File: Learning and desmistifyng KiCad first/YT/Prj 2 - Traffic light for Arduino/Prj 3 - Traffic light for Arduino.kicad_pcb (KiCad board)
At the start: 2 copper layers, 36 x 50.5 mm, 11 parts, among them J2 Conn_01x04

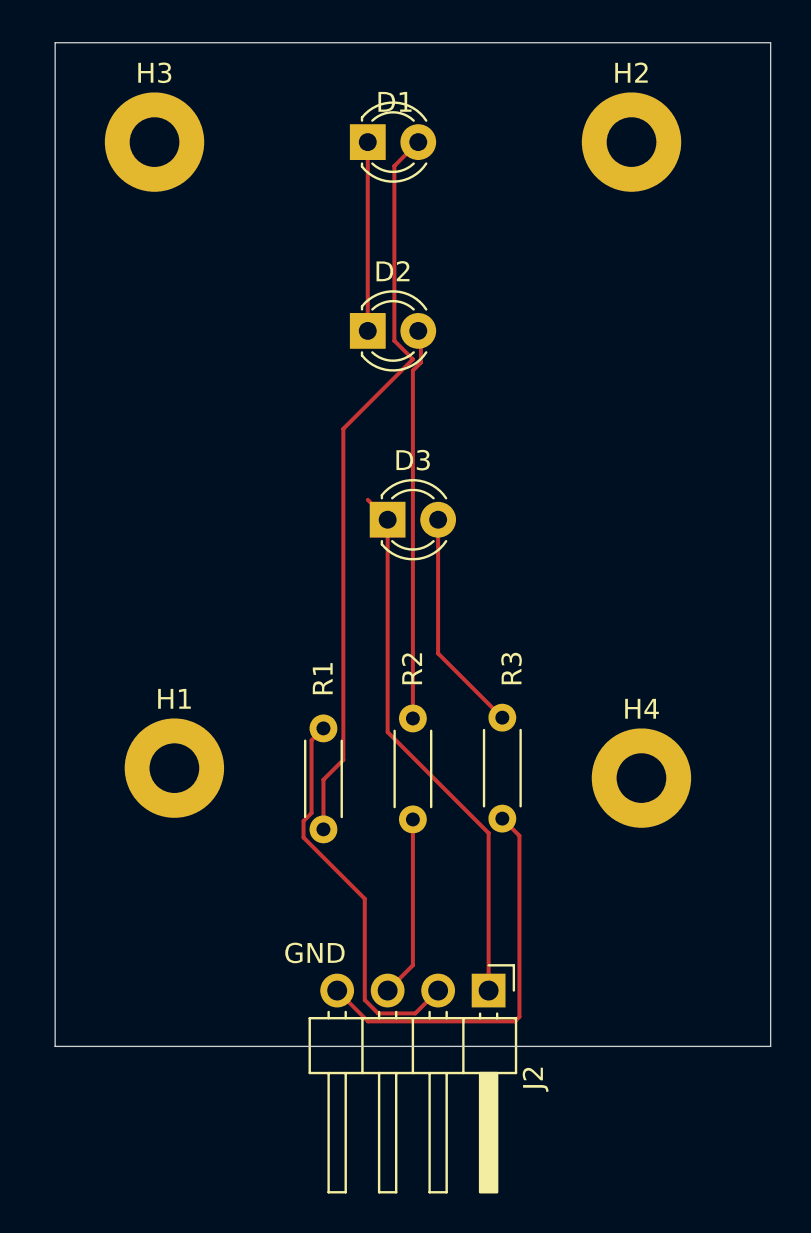
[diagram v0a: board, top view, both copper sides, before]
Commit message: updates on demistifying kicad
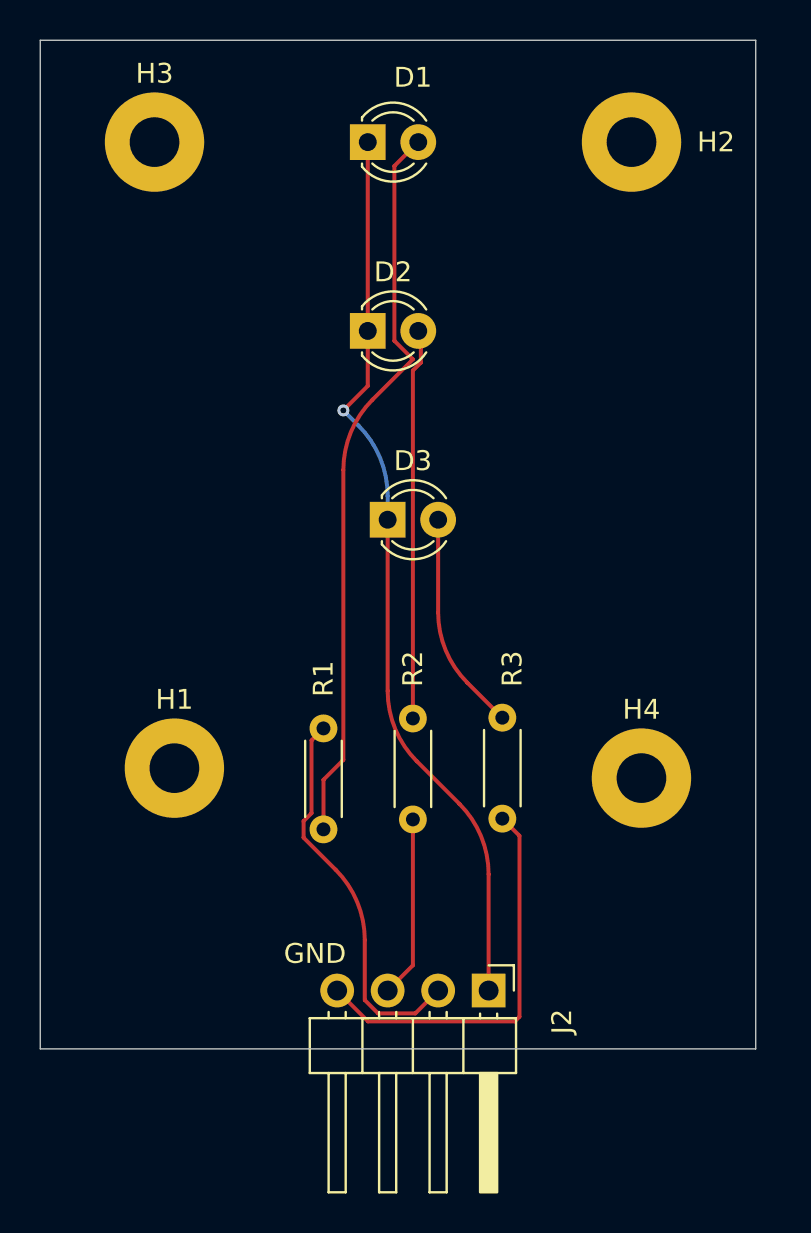
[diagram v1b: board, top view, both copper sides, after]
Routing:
- net Net-(D1-K): track 36.7 -> 45.5 mm, vias 0 -> 1
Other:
- board size 36 x 50.5 mm -> 36 x 50.8 mm
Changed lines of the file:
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@@
 		(tags "mountinghole")
 		(property "Reference" "H2"
-			(at 0 -3.45 0)
+			(at 4.25 0 0)
 			(layer "F.SilkS")
 			(effects
@@
 		)
 		(property "Value" "MountingHole"
-			(at 0 3.45 0)
+			(at 0.25 3.75 0)
 			(layer "F.Fab")
 			(effects
@@
 		)
 		(fp_text user "${REFERENCE}"
-			(at 0 0 0)
+			(at -3.25 2 0)
 			(layer "F.Fab")
 			(effects
@@
 		(tags "LED")
 		(property "Reference" "D1"
-			(at 1.36566 -1.987699 0)
+			(at 2.27 -3.25 0)
 			(layer "F.SilkS")
 			(effects
@@
 		(tags "Through hole angled pin header THT 1x04 2.54mm single row")
 		(property "Reference" "J2"
-			(at 4.385 -2.27 90)
+			(at 1.56 -3.69 90)
 			(layer "F.SilkS")
 			(effects
@@
 			)
 			(layer "F.Fab")
-		)
-		(fp_text user "${REFERENCE}"
-			(at 2.77 3.81 0)
-			(layer "F.Fab")
-			(effects
-				(font
-					(size 1 1)
-					(thickness 0.15)
-				)
-			)
 		)
 		(pad "1" thru_hole rect
@@
 	)
 	(gr_rect
-		(start 160 42.5)
-		(end 196 93)
+		(start 159.25 42.375)
+		(end 195.25 93.125)
 		(stroke
 			(width 0.05)
@@
 	)
 	(segment
-		(start 174.501 61.927471)
+		(start 175.965466 60.463005)
 		(end 178 58.428471)
 		(width 0.2)
@@
 	(segment
 		(start 174.501 78.583372)
-		(end 174.501 61.927471)
+		(end 174.501 63.998539)
 		(width 0.2)
 		(layer "F.Cu")
 		(net 1)
 	)
-	(segment
-		(start 181.81 82.265628)
-		(end 176.73 77.185628)
+	(arc
+		(start 174.501 63.998539)
+		(mid 174.881602 62.085122)
+		(end 175.965466 60.463005)
+		(width 0.2)
+		(layer "F.Cu")
+		(net 1)
+	)
+	(segment
+		(start 180.345534 80.801162)
+		(end 178.194466 78.650094)
 		(width 0.2)
 		(layer "F.Cu")
@@
 	)
 	(segment
-		(start 175.73 65.5)
+		(start 181.81 90.19)
+		(end 181.81 84.336696)
+		(width 0.2)
+		(layer "F.Cu")
+		(net 2)
+	)
+	(segment
+		(start 175.73 59.77)
+		(end 174.5 61)
+		(width 0.2)
+		(layer "F.Cu")
+		(net 2)
+	)
+	(segment
+		(start 175.73 57)
+		(end 175.73 59.77)
+		(width 0.2)
+		(layer "F.Cu")
+		(net 2)
+	)
+	(segment
+		(start 176.73 75.11456)
 		(end 176.73 66.5)
 		(width 0.2)
@@
 		(net 2)
 	)
-	(segment
-		(start 181.81 90.19)
-		(end 181.81 82.265628)
-		(width 0.2)
-		(layer "F.Cu")
+	(via
+		(at 174.5 61)
+		(size 0.6)
+		(drill 0.3)
+		(layers "F.Cu" "B.Cu")
 		(net 2)
 	)
-	(segment
-		(start 176.73 77.185628)
+	(arc
+		(start 180.345534 80.801162)
+		(mid 181.429398 82.423279)
+		(end 181.81 84.336696)
+		(width 0.2)
+		(layer "F.Cu")
+		(net 2)
+	)
+	(arc
+		(start 176.73 75.11456)
+		(mid 177.110602 77.027977)
+		(end 178.194466 78.650094)
+		(width 0.2)
+		(layer "F.Cu")
+		(net 2)
+	)
+	(segment
+		(start 174.5 61)
+		(end 175.265534 61.765534)
+		(width 0.2)
+		(layer "B.Cu")
+		(net 2)
+	)
+	(segment
+		(start 176.73 65.301068)
 		(end 176.73 66.5)
 		(width 0.2)
-		(layer "F.Cu")
+		(layer "B.Cu")
+		(net 2)
+	)
+	(arc
+		(start 176.73 65.301068)
+		(mid 176.349398 63.387651)
+		(end 175.265534 61.765534)
+		(width 0.2)
+		(layer "B.Cu")
 		(net 2)
 	)
@@
 	)
 	(segment
-		(start 179.27 73.23)
+		(start 180.734466 74.694466)
 		(end 182.5 76.46)
 		(width 0.2)
@@
 	(segment
 		(start 179.27 66.5)
-		(end 179.27 73.23)
+		(end 179.27 71.158932)
+		(width 0.2)
+		(layer "F.Cu")
+		(net 4)
+	)
+	(arc
+		(start 180.734466 74.694466)
+		(mid 179.650602 73.072349)
+		(end 179.27 71.158932)
 		(width 0.2)
 		(layer "F.Cu")
@@
 	)
 	(segment
-		(start 175.579 85.574628)
+		(start 174.114534 84.110162)
 		(end 172.499 82.494628)
 		(width 0.2)
@@
 	(segment
 		(start 175.579 90.66676)
-		(end 175.579 85.574628)
-		(width 0.2)
-		(layer "F.Cu")
+		(end 175.579 87.645696)
+		(width 0.2)
+		(layer "F.Cu")
+		(net 6)
+	)
+	(arc
+		(start 174.114534 84.110162)
+		(mid 175.198398 85.732279)
+		(end 175.579 87.645696)
+		(width 0.2)
+		(layer "F.Cu")
